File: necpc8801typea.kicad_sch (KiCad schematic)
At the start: 265 parts, among them J1 Conn_01x01, J2 Conn_01x06, J4 Conn_01x04, Q1 Q_PMOS_GSD AO3401A, Q2 Q_NMOS_GSD 2N7002, Q3 Q_NMOS_GSD 2N7002, SW1 SW_Push, U1 AMS1117-3.3, U2 TPS2553DBVR, U3 STM32F401RETx, U4 24LC64, U5 USBLC6-2SC6, Y1 16MHz

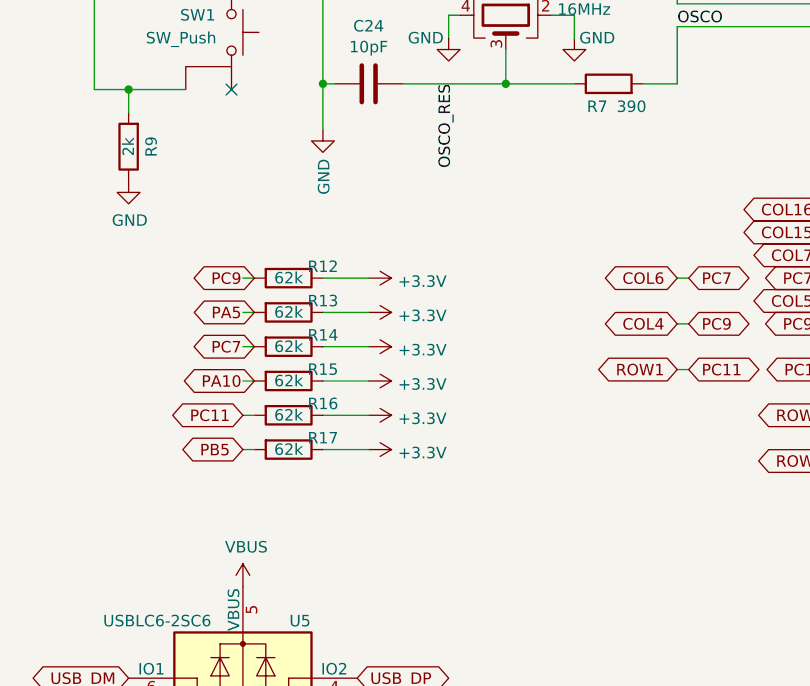
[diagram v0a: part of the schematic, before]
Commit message: updates
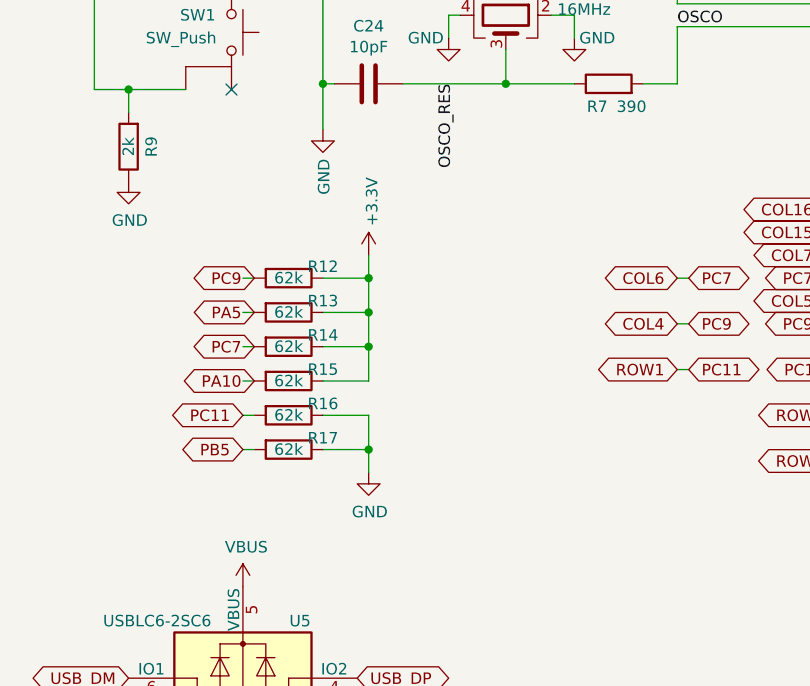
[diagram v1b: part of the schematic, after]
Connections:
- net +3.3VA: no longer R16.1, R17.1
- net GND: now also R16.1, R17.1
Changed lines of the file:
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@@
   (junction (at 121.92 26.67) (diameter 0) (color 0 0 0 0)
   )
+  (junction (at 73.66 158.75) (diameter 0) (color 0 0 0 0)
+  )
   (junction (at 213.36 107.315) (diameter 0) (color 0 0 0 0)
   )
@@
   (junction (at 91.44 243.84) (diameter 1.016) (color 0 0 0 0)
   )
+  (junction (at 73.66 147.32) (diameter 0) (color 0 0 0 0)
+  )
   (junction (at 330.2 273.05) (diameter 0) (color 0 0 0 0)
   )
@@
   (junction (at 233.68 281.94) (diameter 1.016) (color 0 0 0 0)
   )
+  (junction (at 73.66 139.7) (diameter 0) (color 0 0 0 0)
+  )
   (junction (at 127 243.84) (diameter 1.016) (color 0 0 0 0)
   )
@@
   (junction (at 57.15 243.84) (diameter 1.016) (color 0 0 0 0)
   )
+  (junction (at 73.66 143.51) (diameter 0) (color 0 0 0 0)
+  )
   (junction (at 278.13 311.15) (diameter 1.016) (color 0 0 0 0)
   )
@@
     (stroke (width 0) (type solid))
   )
+  (wire (pts (xy 73.66 137.16) (xy 73.66 139.7))
+    (stroke (width 0) (type default))
+  )
   (wire (pts (xy 337.82 300.99) (xy 337.82 320.04))
     (stroke (width 0) (type solid))
@@
     (stroke (width 0) (type solid))
   )
+  (wire (pts (xy 73.66 158.75) (xy 73.66 161.29))
+    (stroke (width 0) (type default))
+  )
   (wire (pts (xy 337.82 243.84) (xy 337.82 262.89))
     (stroke (width 0) (type solid))
@@
     (stroke (width 0) (type solid))
   )
+  (wire (pts (xy 73.66 154.94) (xy 73.66 158.75))
+    (stroke (width 0) (type default))
+  )
   (wire (pts (xy 19.685 26.67) (xy 22.86 26.67))
     (stroke (width 0) (type default))
@@
     (stroke (width 0) (type solid))
   )
+  (wire (pts (xy 73.66 143.51) (xy 73.66 147.32))
+    (stroke (width 0) (type default))
+  )
   (wire (pts (xy 171.45 306.07) (xy 173.99 306.07))
     (stroke (width 0) (type solid))
@@
     (stroke (width 0) (type solid))
   )
+  (wire (pts (xy 73.66 139.7) (xy 73.66 143.51))
+    (stroke (width 0) (type default))
+  )
   (wire (pts (xy 226.06 330.2) (xy 242.57 330.2))
     (stroke (width 0) (type solid))
@@
     (stroke (width 0) (type solid))
   )
+  (wire (pts (xy 73.66 147.32) (xy 73.66 151.13))
+    (stroke (width 0) (type default))
+  )
   (wire (pts (xy 355.6 300.99) (xy 355.6 281.94))
     (stroke (width 0) (type solid))
@@
     )
   )
-  (symbol (lib_id "controller-rescue:+3.3V-power") (at 73.66 147.32 270) (unit 1)
-    (in_bom yes) (on_board yes) (dnp no)
-    (property "Reference" "#PWR0118" (at 69.85 147.32 0)
-      (effects (font (size 1.27 1.27)) hide)
-    )
-    (property "Value" "+3.3V" (at 76.9112 147.701 90)
-      (effects (font (size 1.27 1.27)) (justify left))
-    )
-    (property "Footprint" "" (at 73.66 147.32 0)
-      (effects (font (size 1.27 1.27)) hide)
-    )
-    (property "Datasheet" "" (at 73.66 147.32 0)
-      (effects (font (size 1.27 1.27)) hide)
-    )
-    (pin "1")
-    (instances
-      (project "necpc8801typea"
-        (path "/151da08b-0979-4785-a9bf-6fa9b165d629"
-          (reference "#PWR0118") (unit 1)
-        )
-      )
-      (project "controller"
-        (path "/d7b41e20-3ed8-4e20-8d18-95c1ff55bd12"
-          (reference "#PWR0118") (unit 1)
-        )
-      )
-    )
-  )
   (symbol (lib_id "controller-rescue:GND-power") (at 52.07 94.615 0) (unit 1)
     (in_bom yes) (on_board yes) (dnp no)
@@
     )
   )
-  (symbol (lib_id "controller-rescue:+3.3V-power") (at 73.66 154.94 270) (unit 1)
-    (in_bom yes) (on_board yes) (dnp no)
-    (property "Reference" "#PWR0126" (at 69.85 154.94 0)
-      (effects (font (size 1.27 1.27)) hide)
-    )
-    (property "Value" "+3.3V" (at 76.9112 155.321 90)
-      (effects (font (size 1.27 1.27)) (justify left))
-    )
-    (property "Footprint" "" (at 73.66 154.94 0)
-      (effects (font (size 1.27 1.27)) hide)
-    )
-    (property "Datasheet" "" (at 73.66 154.94 0)
-      (effects (font (size 1.27 1.27)) hide)
-    )
-    (pin "1")
-    (instances
-      (project "necpc8801typea"
-        (path "/151da08b-0979-4785-a9bf-6fa9b165d629"
-          (reference "#PWR0126") (unit 1)
-        )
-      )
-      (project "controller"
-        (path "/d7b41e20-3ed8-4e20-8d18-95c1ff55bd12"
-          (reference "#PWR0105") (unit 1)
-        )
-      )
-    )
-  )
   (symbol (lib_id "MX_Alps_Hybrid:mx-alps-nec") (at 334.01 264.16 0) (unit 1)
     (in_bom yes) (on_board yes) (dnp no)
@@
     )
   )
-  (symbol (lib_id "controller-rescue:+3.3V-power") (at 73.66 158.75 270) (unit 1)
-    (in_bom yes) (on_board yes) (dnp no)
-    (property "Reference" "#PWR0127" (at 69.85 158.75 0)
-      (effects (font (size 1.27 1.27)) hide)
-    )
-    (property "Value" "+3.3V" (at 76.9112 159.131 90)
-      (effects (font (size 1.27 1.27)) (justify left))
-    )
-    (property "Footprint" "" (at 73.66 158.75 0)
-      (effects (font (size 1.27 1.27)) hide)
-    )
-    (property "Datasheet" "" (at 73.66 158.75 0)
-      (effects (font (size 1.27 1.27)) hide)
-    )
-    (pin "1")
-    (instances
-      (project "necpc8801typea"
-        (path "/151da08b-0979-4785-a9bf-6fa9b165d629"
-          (reference "#PWR0127") (unit 1)
-        )
-      )
-      (project "controller"
-        (path "/d7b41e20-3ed8-4e20-8d18-95c1ff55bd12"
-          (reference "#PWR0105") (unit 1)
-        )
-      )
-    )
-  )
   (symbol (lib_id "controller-rescue:GND-power") (at 99.06 94.615 0) (unit 1)
     (in_bom yes) (on_board yes) (dnp no)
@@
     )
   )
-  (symbol (lib_id "controller-rescue:+3.3V-power") (at 73.66 151.13 270) (unit 1)
-    (in_bom yes) (on_board yes) (dnp no)
-    (property "Reference" "#PWR0105" (at 69.85 151.13 0)
-      (effects (font (size 1.27 1.27)) hide)
-    )
-    (property "Value" "+3.3V" (at 76.9112 151.511 90)
-      (effects (font (size 1.27 1.27)) (justify left))
-    )
-    (property "Footprint" "" (at 73.66 151.13 0)
-      (effects (font (size 1.27 1.27)) hide)
-    )
-    (property "Datasheet" "" (at 73.66 151.13 0)
-      (effects (font (size 1.27 1.27)) hide)
-    )
-    (pin "1")
-    (instances
-      (project "necpc8801typea"
-        (path "/151da08b-0979-4785-a9bf-6fa9b165d629"
-          (reference "#PWR0105") (unit 1)
-        )
-      )
-      (project "controller"
-        (path "/d7b41e20-3ed8-4e20-8d18-95c1ff55bd12"
-          (reference "#PWR0105") (unit 1)
-        )
-      )
-    )
-  )
   (symbol (lib_id "Device:D_Small") (at 347.98 308.61 90) (unit 1)
     (in_bom yes) (on_board yes) (dnp no)
@@
     )
   )
-  (symbol (lib_id "controller-rescue:+3.3V-power") (at 73.66 139.7 270) (unit 1)
+  (symbol (lib_id "controller-rescue:+3.3V-power") (at 73.66 137.16 0) (unit 1)
     (in_bom yes) (on_board yes) (dnp no)
-    (property "Reference" "#PWR0116" (at 69.85 139.7 0)
+    (property "Reference" "#PWR0116" (at 73.66 140.97 0)
       (effects (font (size 1.27 1.27)) hide)
     )
-    (property "Value" "+3.3V" (at 76.9112 140.081 90)
+    (property "Value" "+3.3V" (at 74.041 133.9088 90)
       (effects (font (size 1.27 1.27)) (justify left))
     )
-    (property "Footprint" "" (at 73.66 139.7 0)
+    (property "Footprint" "" (at 73.66 137.16 0)
       (effects (font (size 1.27 1.27)) hide)
     )
-    (property "Datasheet" "" (at 73.66 139.7 0)
+    (property "Datasheet" "" (at 73.66 137.16 0)
       (effects (font (size 1.27 1.27)) hide)
     )
@@
     )
   )
-  (symbol (lib_id "controller-rescue:+3.3V-power") (at 73.66 143.51 270) (unit 1)
-    (in_bom yes) (on_board yes) (dnp no)
-    (property "Reference" "#PWR0117" (at 69.85 143.51 0)
-      (effects (font (size 1.27 1.27)) hide)
-    )
-    (property "Value" "+3.3V" (at 76.9112 143.891 90)
-      (effects (font (size 1.27 1.27)) (justify left))
-    )
-    (property "Footprint" "" (at 73.66 143.51 0)
-      (effects (font (size 1.27 1.27)) hide)
-    )
-    (property "Datasheet" "" (at 73.66 143.51 0)
-      (effects (font (size 1.27 1.27)) hide)
-    )
-    (pin "1")
-    (instances
-      (project "necpc8801typea"
-        (path "/151da08b-0979-4785-a9bf-6fa9b165d629"
-          (reference "#PWR0117") (unit 1)
-        )
-      )
-      (project "controller"
-        (path "/d7b41e20-3ed8-4e20-8d18-95c1ff55bd12"
-          (reference "#PWR0117") (unit 1)
-        )
-      )
-    )
-  )
   (symbol (lib_id "Device:R") (at 64.77 139.7 270) (unit 1)
     (in_bom yes) (on_board yes) (dnp no)
@@
         )
       )
+    )
+  )
+  (symbol (lib_id "controller-rescue:GND-power") (at 73.66 161.29 0) (unit 1)
+    (in_bom yes) (on_board yes) (dnp no)
+    (property "Reference" "#PWR035" (at 73.66 167.64 0)
+      (effects (font (size 1.27 1.27)) hide)
+    )
+    (property "Value" "GND" (at 73.787 165.6842 0)
+      (effects (font (size 1.27 1.27)))
+    )
+    (property "Footprint" "" (at 73.66 161.29 0)
+      (effects (font (size 1.27 1.27)) hide)
+    )
+    (property "Datasheet" "" (at 73.66 161.29 0)
+      (effects (font (size 1.27 1.27)) hide)
+    )
+    (pin "1")
+    (instances
+      (project "necpc8801typea"
+        (path "/151da08b-0979-4785-a9bf-6fa9b165d629"
+          (reference "#PWR035") (unit 1)
+        )
+      )
+      (project "controller"
+        (path "/d7b41e20-3ed8-4e20-8d18-95c1ff55bd12"
+          (reference "#PWR035") (unit 1)
+        )
+      )

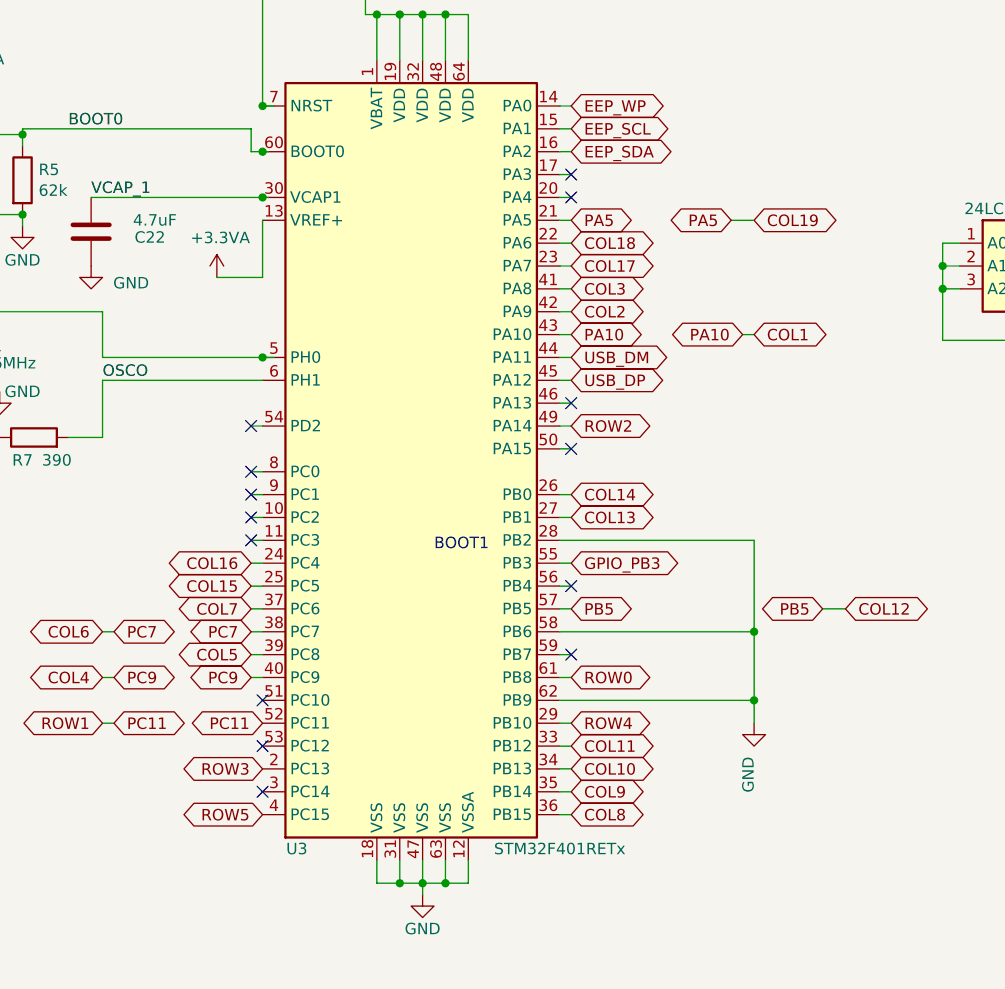
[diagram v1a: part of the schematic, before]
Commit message: updates
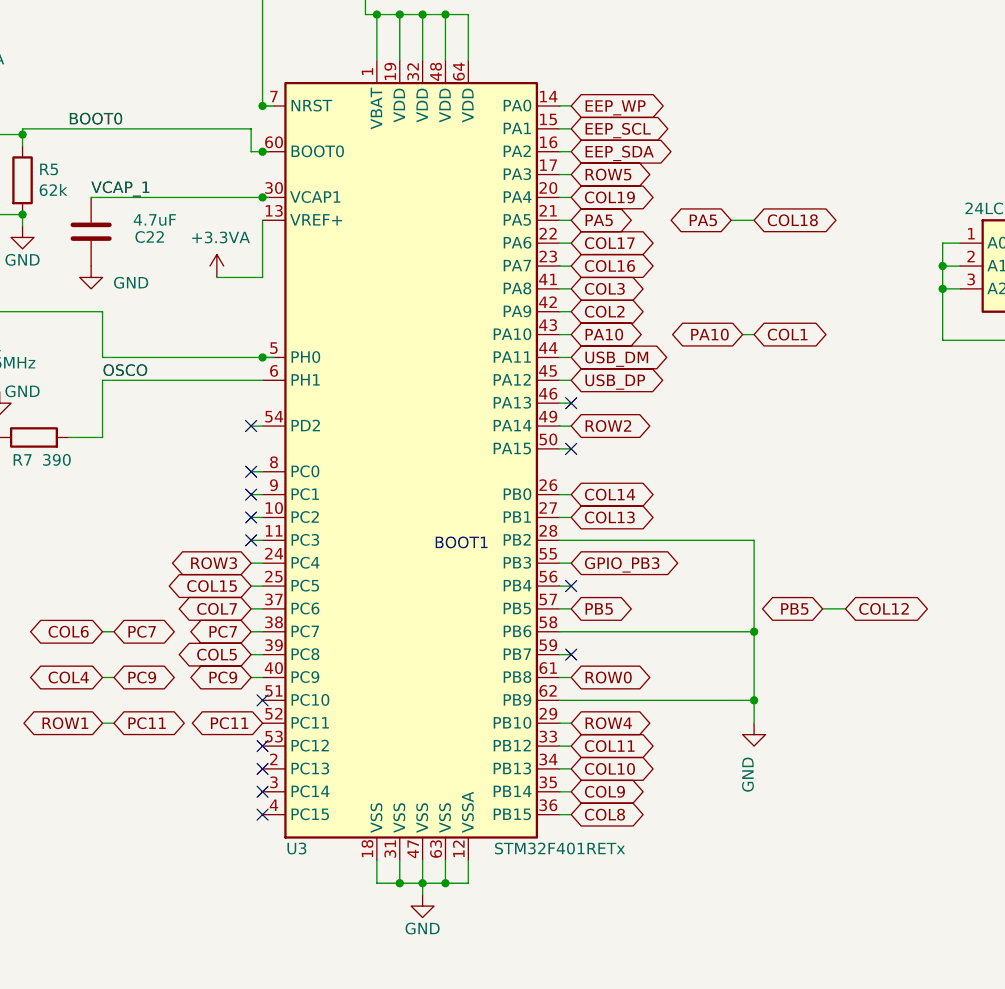
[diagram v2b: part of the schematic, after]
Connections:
- net COL16: now also U3.23 (PA7); no longer U3.24 (PC4)
- net COL17: now also U3.22 (PA6); no longer U3.23 (PA7)
- net COL18: now also R13.2, U3.21 (PA5); no longer U3.22 (PA6)
- net COL19: now also U3.20 (PA4); no longer R13.2, U3.21 (PA5)
- net ROW3: now also U3.24 (PC4); no longer U3.2 (PC13)
- net ROW5: now also U3.17 (PA3); no longer U3.4 (PC15)
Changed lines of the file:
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@@
   (no_connect (at 58.42 118.745))
   (no_connect (at 125.73 147.32))
-  (no_connect (at 160.02 91.44))
+  (no_connect (at 125.73 160.02))
   (no_connect (at 124.46 121.92))
   (no_connect (at 124.46 124.46))
@@
   (no_connect (at 160.02 114.3))
   (no_connect (at 125.73 157.48))
-  (no_connect (at 160.02 88.9))
+  (no_connect (at 125.73 154.94))
   (no_connect (at 53.34 106.045))
   (wire (pts (xy 107.95 118.11) (xy 104.14 118.11))
@@
     (stroke (width 0) (type solid))
   )
-  (wire (pts (xy 158.75 91.44) (xy 160.02 91.44))
-    (stroke (width 0) (type default))
-  )
   (wire (pts (xy 180.34 129.54) (xy 180.34 139.7))
     (stroke (width 0) (type default))
@@
     (stroke (width 0) (type default))
   )
+  (wire (pts (xy 158.75 91.44) (xy 160.02 91.44))
+    (stroke (width 0) (type default))
+  )
   (wire (pts (xy 31.75 306.07) (xy 34.29 306.07))
     (stroke (width 0) (type solid))
@@
     )
   )
-  (global_label "ROW5" (shape bidirectional) (at 125.73 160.02 180)
-    (effects (font (size 1.27 1.27)) (justify right))
-    (property "Intersheetrefs" "${INTERSHEET_REFS}" (at 125.73 160.02 0)
+  (global_label "ROW5" (shape bidirectional) (at 160.02 88.9 0)
+    (effects (font (size 1.27 1.27)) (justify left))
+    (property "Intersheetrefs" "${INTERSHEET_REFS}" (at 160.02 88.9 0)
       (effects (font (size 1.27 1.27)) hide)
     )
@@
     )
   )
-  (global_label "COL16" (shape bidirectional) (at 124.46 132.08 180)
-    (effects (font (size 1.27 1.27)) (justify right))
-    (property "Intersheetrefs" "${INTERSHEET_REFS}" (at 124.46 132.08 0)
+  (global_label "COL16" (shape bidirectional) (at 160.02 99.06 0)
+    (effects (font (size 1.27 1.27)) (justify left))
+    (property "Intersheetrefs" "${INTERSHEET_REFS}" (at 160.02 99.06 0)
       (effects (font (size 1.27 1.27)) hide)
     )
@@
     )
   )
-  (global_label "COL17" (shape bidirectional) (at 160.02 99.06 0)
+  (global_label "COL17" (shape bidirectional) (at 160.02 96.52 0)
     (effects (font (size 1.27 1.27)) (justify left))
-    (property "Intersheetrefs" "${INTERSHEET_REFS}" (at 160.02 99.06 0)
+    (property "Intersheetrefs" "${INTERSHEET_REFS}" (at 160.02 96.52 0)
       (effects (font (size 1.27 1.27)) hide)
     )
@@
     )
   )
-  (global_label "ROW3" (shape bidirectional) (at 125.73 154.94 180)
+  (global_label "ROW3" (shape bidirectional) (at 124.46 132.08 180)
     (effects (font (size 1.27 1.27)) (justify right))
-    (property "Intersheetrefs" "${INTERSHEET_REFS}" (at 125.73 154.94 0)
+    (property "Intersheetrefs" "${INTERSHEET_REFS}" (at 124.46 132.08 0)
       (effects (font (size 1.27 1.27)) hide)
     )
@@
     )
   )
-  (global_label "COL18" (shape bidirectional) (at 160.02 96.52 0)
+  (global_label "COL18" (shape bidirectional) (at 180.34 93.98 0)
     (effects (font (size 1.27 1.27)) (justify left))
-    (property "Intersheetrefs" "${INTERSHEET_REFS}" (at 160.02 96.52 0)
+    (property "Intersheetrefs" "${INTERSHEET_REFS}" (at 180.34 93.98 0)
       (effects (font (size 1.27 1.27)) hide)
     )
@@
     )
   )
-  (global_label "COL19" (shape bidirectional) (at 180.34 93.98 0)
+  (global_label "COL19" (shape bidirectional) (at 160.02 91.44 0)
     (effects (font (size 1.27 1.27)) (justify left))
-    (property "Intersheetrefs" "${INTERSHEET_REFS}" (at 180.34 93.98 0)
+    (property "Intersheetrefs" "${INTERSHEET_REFS}" (at 160.02 91.44 0)
       (effects (font (size 1.27 1.27)) hide)
     )
@@
   (symbol (lib_id "controller-rescue:GND-power") (at 46.99 128.905 0) (unit 1)
     (in_bom yes) (on_board yes) (dnp no)
-    (property "Reference" "#PWR035" (at 46.99 135.255 0)
+    (property "Reference" "#PWR0105" (at 46.99 135.255 0)
       (effects (font (size 1.27 1.27)) hide)
     )
@@
       (project "necpc8801typea"
         (path "/151da08b-0979-4785-a9bf-6fa9b165d629"
-          (reference "#PWR035") (unit 1)
+          (reference "#PWR0105") (unit 1)
         )
       )
